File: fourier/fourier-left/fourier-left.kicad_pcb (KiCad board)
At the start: 2 copper layers, 124.4 x 84.6 mm, 125 parts, among them J1 VCC, J3 RGB, J6 C6, J7 GND, U1 ProMicro, U2 TRRS

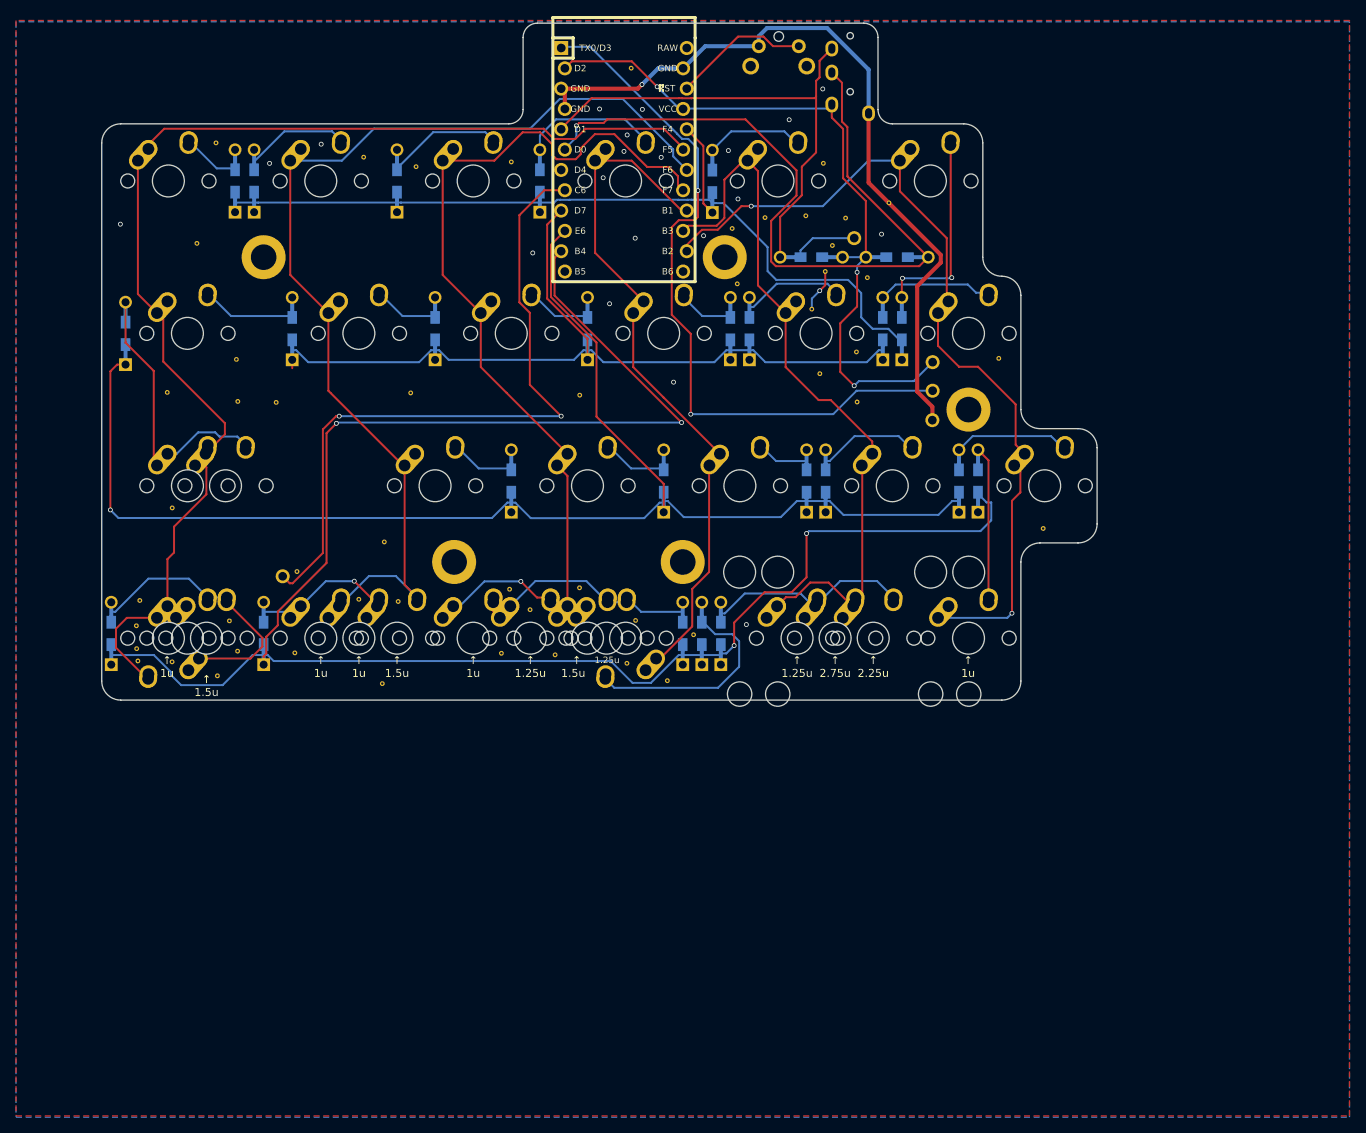
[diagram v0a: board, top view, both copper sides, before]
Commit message: rotate left-top and update to KiCad 5.99
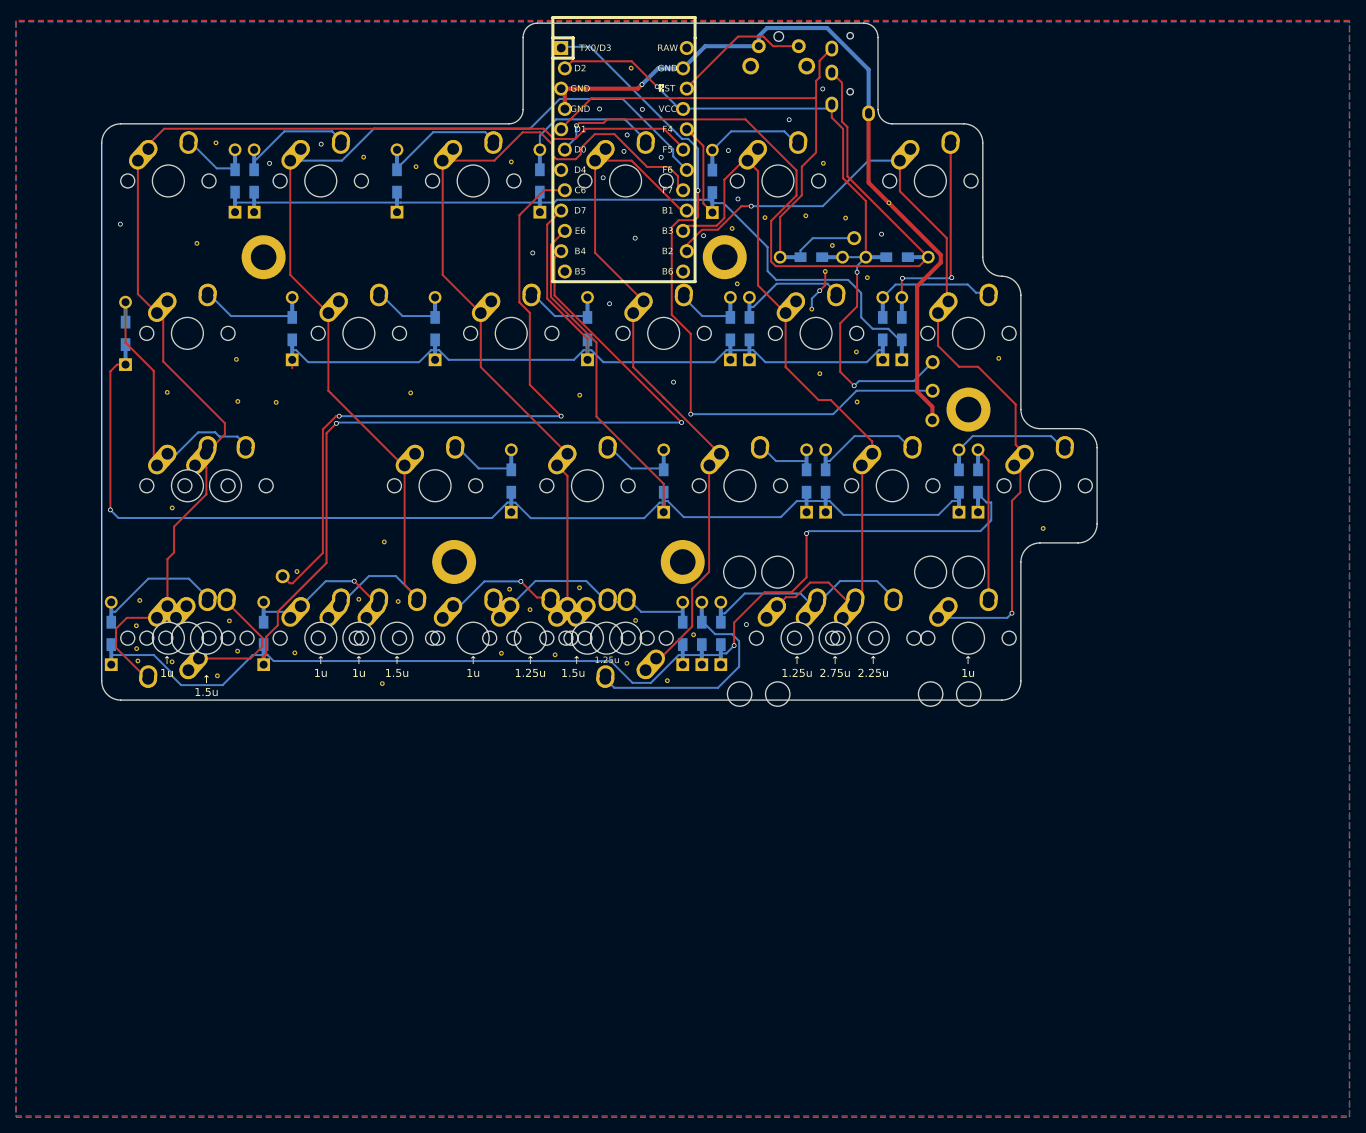
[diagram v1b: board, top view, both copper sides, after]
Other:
- net class Default removed
- net class Power removed
